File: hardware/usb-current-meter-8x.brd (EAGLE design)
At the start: 78.5 x 29.2 mm, 39 parts, among them IC3 MEGA48/88/168-AU, IC9 OPA2234U, X7 MC2

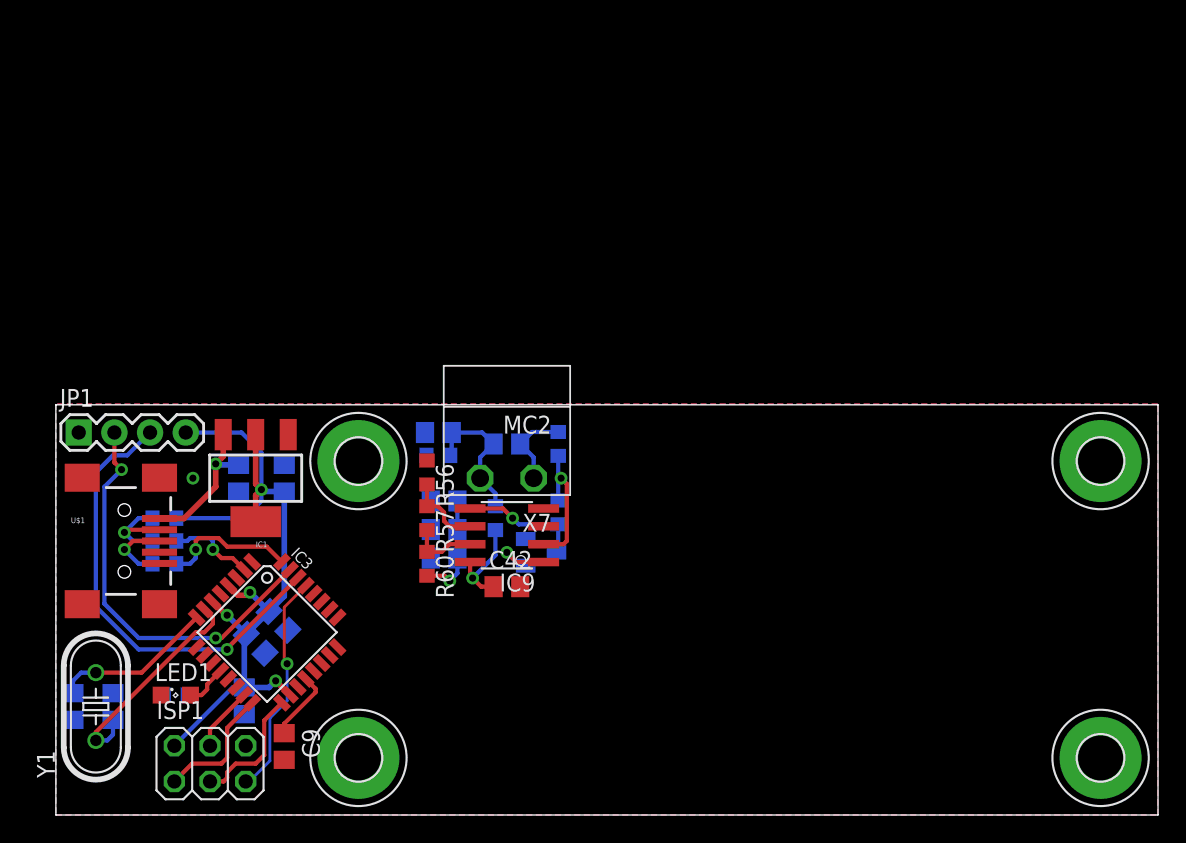
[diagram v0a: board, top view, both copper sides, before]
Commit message: hardware: progress save
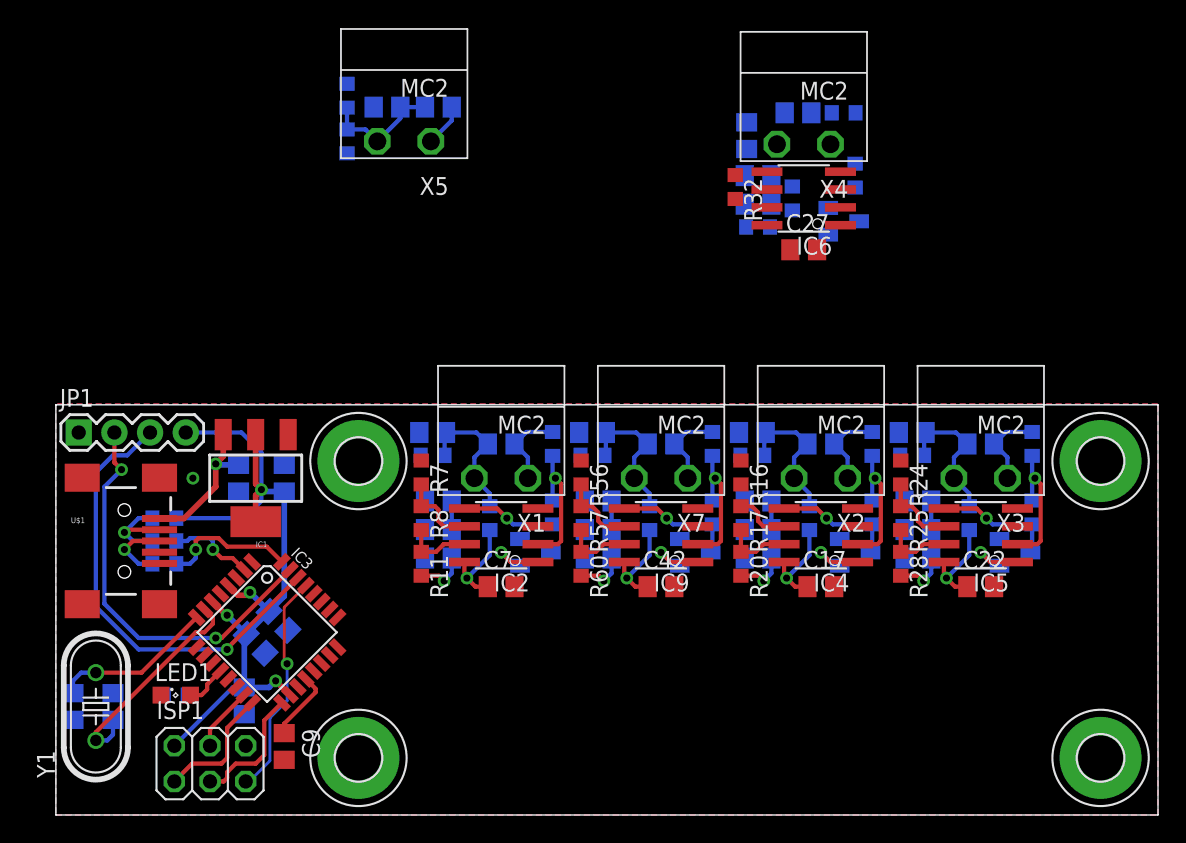
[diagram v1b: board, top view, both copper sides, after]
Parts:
- added C14, C17, C19, C22, C27, C29, C4, C7: 100n, rcl:C0805
- added C15, C16, C18, C20, C21, C23, C25, C26, C28, C5, C6, C8: 1u, rcl:C0805
- added D1, D2, D3, D4: BAT54, diode:SOT23
- added IC2, IC4, IC5, IC6: OPA2234U, burr-brown:SO08
- added R10, R14, R15, R16, R17, R18, R19, R22, R23, R24, R25, R26, R27, R30, R31, R32, R33, R42, R43, R5, R6, R7, R8, R9: tbd, rcl:R0603
- added R11, R20, R28, R36: 100k, rcl:R0603
- added R12, R21, R29, R37, R4: Rload, rcl:R0805
- added X1, X2, X3, X4, X5: MC2, con-phoenix-381_l:MC2
- moved D7 11.0 mm to (45.5, 18.7)
- moved R56 11.0 mm to (37.4, 24.4)
- moved R57 11.0 mm to (37.4, 21.1)
- moved R60 11.0 mm to (37.4, 17.9)
- moved C39 11.0 mm to (38.2, 27.2)
- moved C42 11.0 mm to (43.1, 16.3)
- moved IC9 11.0 mm to (43.1, 19.9)
- moved R53 11.0 mm to (43.1, 26.4)
- moved R54 11.0 mm to (46.7, 26.4)
- moved R55 11.0 mm to (46.7, 21.5)
- moved R58 11.0 mm to (42.3, 21.1)
- moved R59 11.0 mm to (38.2, 25.6)
- moved X7 11.0 mm to (43.1, 24.0)
- moved C40 11.0 mm to (38.6, 20.3)
- moved C41 11.0 mm to (38.6, 22.4)
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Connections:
- net SC_IN_B renamed SC_IN_B_0
- removed net SC_IN_A: R53.2, R54.1, X7.1
- new net N$10: IC2.6, R7.2, R8.1
- new net N$11: IC2.7, R11.1, R8.2
- new net N$12: IC4.2, R14.2, R15.1
- new net N$13: D2.1, IC4.1
- new net N$14: D2.3, IC4.5, R15.2
- new net N$15: IC4.6, R16.2, R17.1
- new net N$16: IC4.7, R17.2, R20.1
- new net N$17: IC6.2, R30.2, R31.1
- new net N$18: D4.1, IC6.1
- new net N$19: D4.3, IC6.5, R31.2
- new net N$20: IC6.6, R32.2, R33.1
- new net N$21: IC6.7, R33.2, R36.1
- new net N$22: IC5.2, R22.2, R23.1
- new net N$23: D3.1, IC5.1
- new net N$24: D3.3, IC5.5, R23.2
- new net N$25: IC5.6, R24.2, R25.1
- new net N$26: IC5.7, R25.2, R28.1
- new net N$7: IC2.2, R5.2, R6.1
- new net N$8: D1.1, IC2.1
- new net N$9: D1.3, IC2.5, R6.2
- new net SC_IN_A_0: R29.2, R30.1, R53.2, R54.1, X4.1, X7.1
- new net SC_IN_A_1: R4.2, R5.1, X1.1
- new net SC_IN_A_2: R12.2, R14.1, X2.1
- new net SC_IN_A_3: R21.2, R22.1, X3.1
- new net SC_IN_B_1: C4.1, R10.2, R4.1, R9.1, X1.2
- new net SC_IN_B_2: C14.1, R12.1, R18.1, R19.2, X2.2
- new net SC_IN_B_3: C19.1, R21.1, R26.1, R27.2, X3.2
- new net SC_IN_B_5: C29.1, R37.1, R42.1, R43.2, X5.2
- net GND: now also C14.2, C15.2, C16.2, C17.2, C18.2, C19.2, C20.2, C21.2, C22.2, C23.2, C25.2, C26.2, C27.2, C28.2, C29.2, C4.2, C5.2, C6.2, C7.2, C8.2, IC2.3, IC2.4, IC4.3, IC4.4, IC5.3, IC5.4, IC6.3, IC6.4, R10.1, R16.1, R19.1, R24.1, R27.1, R29.1, R32.1, R43.1, R7.1, X4.2
- net IN_CH0: now also C25.1, C26.1, C28.1, R36.2
- net IN_CH1: now also C5.1, C6.1, C8.1, R11.2, R37.2, X5.1
- net IN_CH2: now also C15.1, C16.1, C18.1, R20.2
- net IN_CH3: now also C20.1, C21.1, C23.1, R28.2
- net VCC: now also C17.1, C22.1, C27.1, C7.1, IC2.8, IC4.8, IC5.8, IC6.8, R18.2, R26.2, R42.2, R9.2
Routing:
- net VCC: track 64.1 -> 85.3 mm, vias 5 -> 7
- net IN_CH1: track 0.00 -> 10.7 mm, vias 0 -> 1
- net SC_IN_B_2: track 0.00 -> 10.3 mm
- net SC_IN_B_1: track 0.00 -> 10.3 mm
- net SC_IN_B_3: track 0.00 -> 10.3 mm
- net N$7: track 0.00 -> 9.73 mm, vias 0 -> 1
- net N$12: track 0.00 -> 9.73 mm, vias 0 -> 1
- net N$22: track 0.00 -> 9.73 mm, vias 0 -> 1
- net SC_IN_B_5: track 0.00 -> 8.94 mm
- net N$14: track 0.00 -> 8.79 mm, vias 0 -> 1
- net N$24: track 0.00 -> 8.79 mm, vias 0 -> 1
- net IN_CH3: track 0.00 -> 7.69 mm, vias 0 -> 1
- net IN_CH2: track 0.00 -> 7.69 mm, vias 0 -> 1
- net N$9: track 0.00 -> 6.74 mm, vias 0 -> 1
- net SC_IN_A_0: track 0.00 -> 5.89 mm
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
